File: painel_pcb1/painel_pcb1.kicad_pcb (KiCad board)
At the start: 2 copper layers, 91.4 x 119.4 mm, 57 parts, among them J1 Conn_02x16_Counter_Clockwise, J2 Conn_02x02_Counter_Clockwise, J3 Conn_02x06_Counter_Clockwise, J4 Conn_02x08_Counter_Clockwise, J5 Conn_02x03_Counter_Clockwise, J6 Conn_02x08_Counter_Clockwise, U1 MAX7219, U2 MAX7219, U3 74LS595, U4 74LS595

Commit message: converted to KICAD 6
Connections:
- net ~RESET renamed ~{RESET}
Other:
- net class Default removed

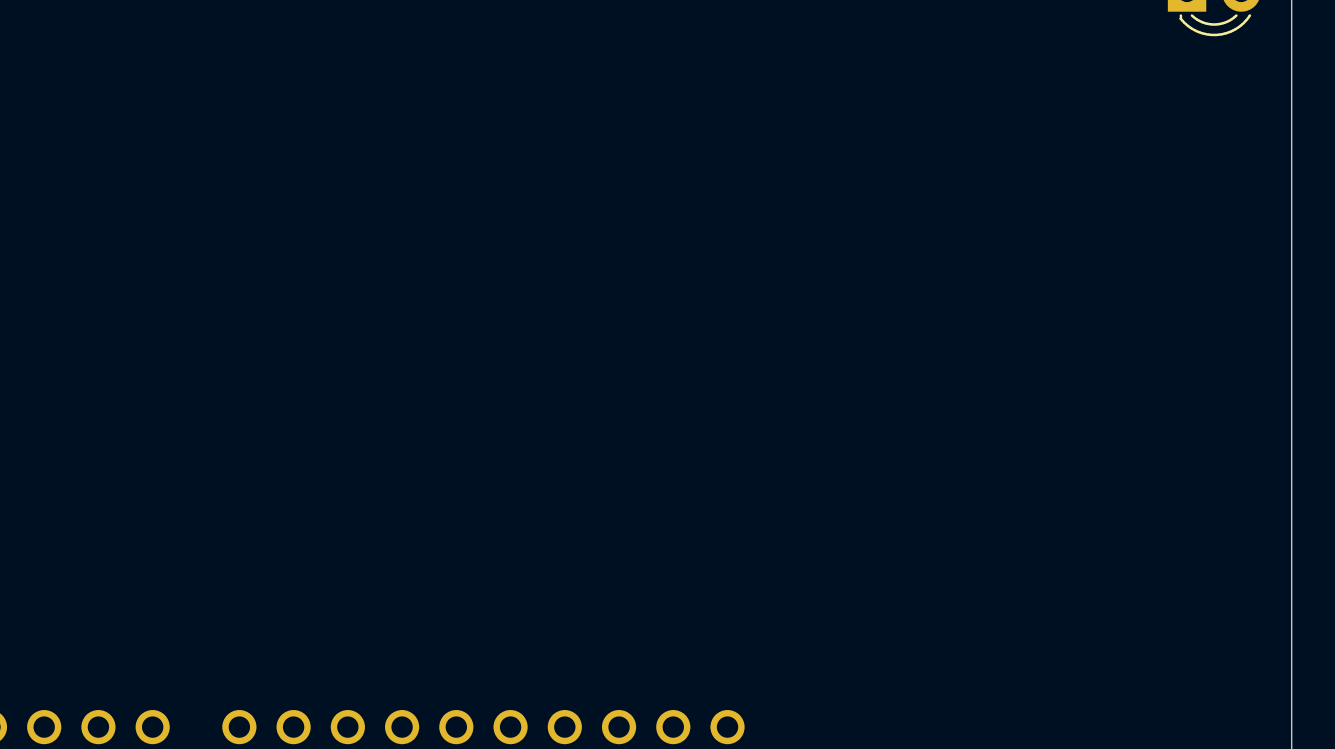
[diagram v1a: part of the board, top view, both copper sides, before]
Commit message: wip
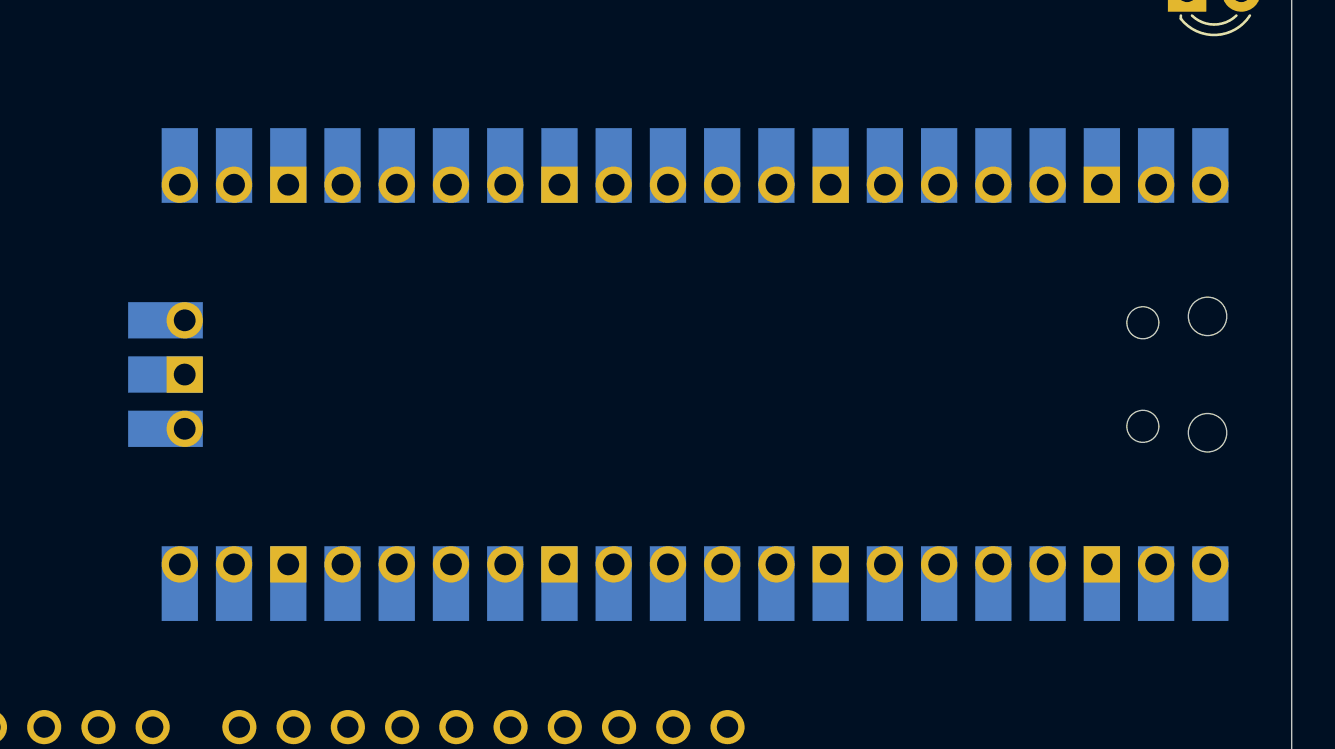
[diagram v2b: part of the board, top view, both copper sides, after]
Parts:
- added U5: Pico, MCU_RaspberryPi_and_Boards:RPi_Pico_SMD_TH, B.Cu at (114.3, 119.4)
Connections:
- A1 pad 1: Net-(A1-Pad1) -> unconnected-(A1-Pad1)
